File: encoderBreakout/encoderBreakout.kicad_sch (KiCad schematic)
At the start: 2 parts, among them J1 Conn_01x08_MountingPin

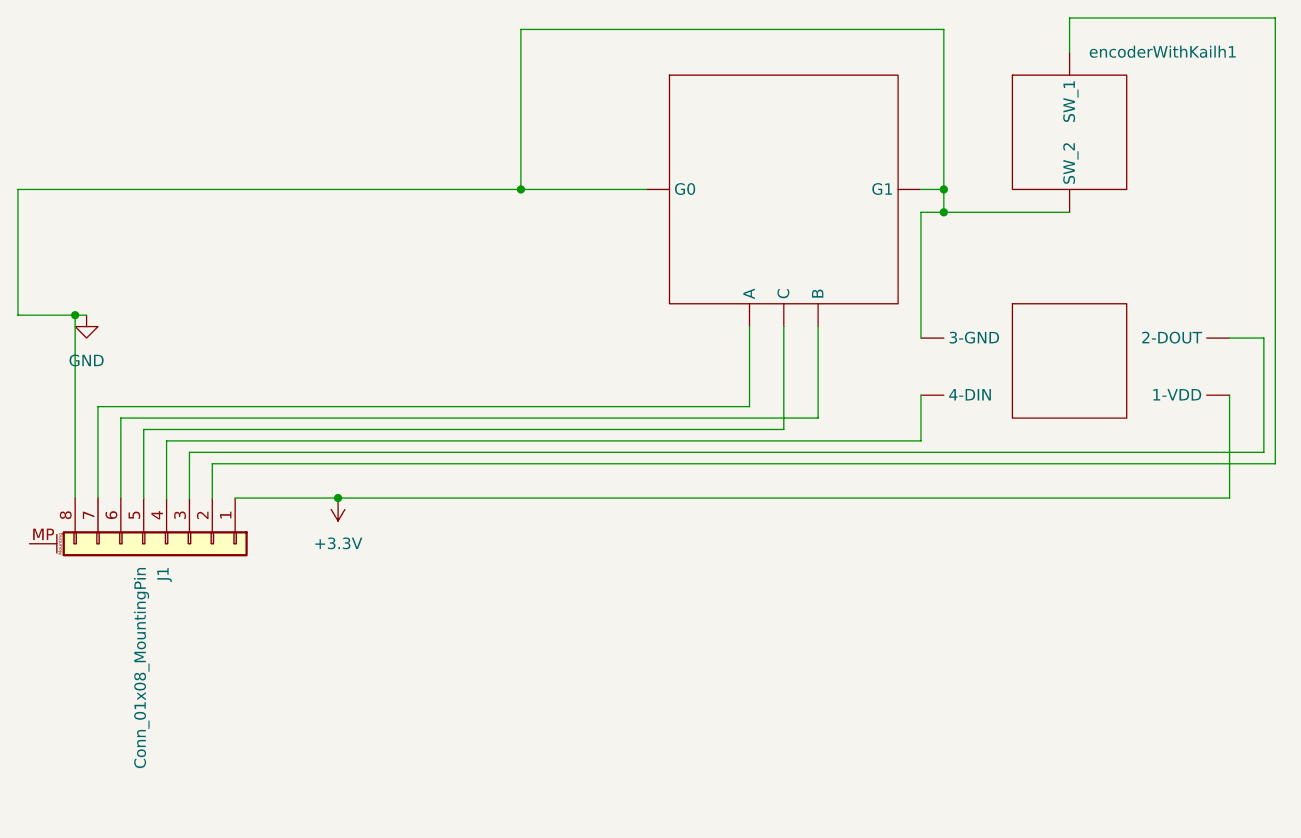
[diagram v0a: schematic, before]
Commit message: encoder breakout rev a
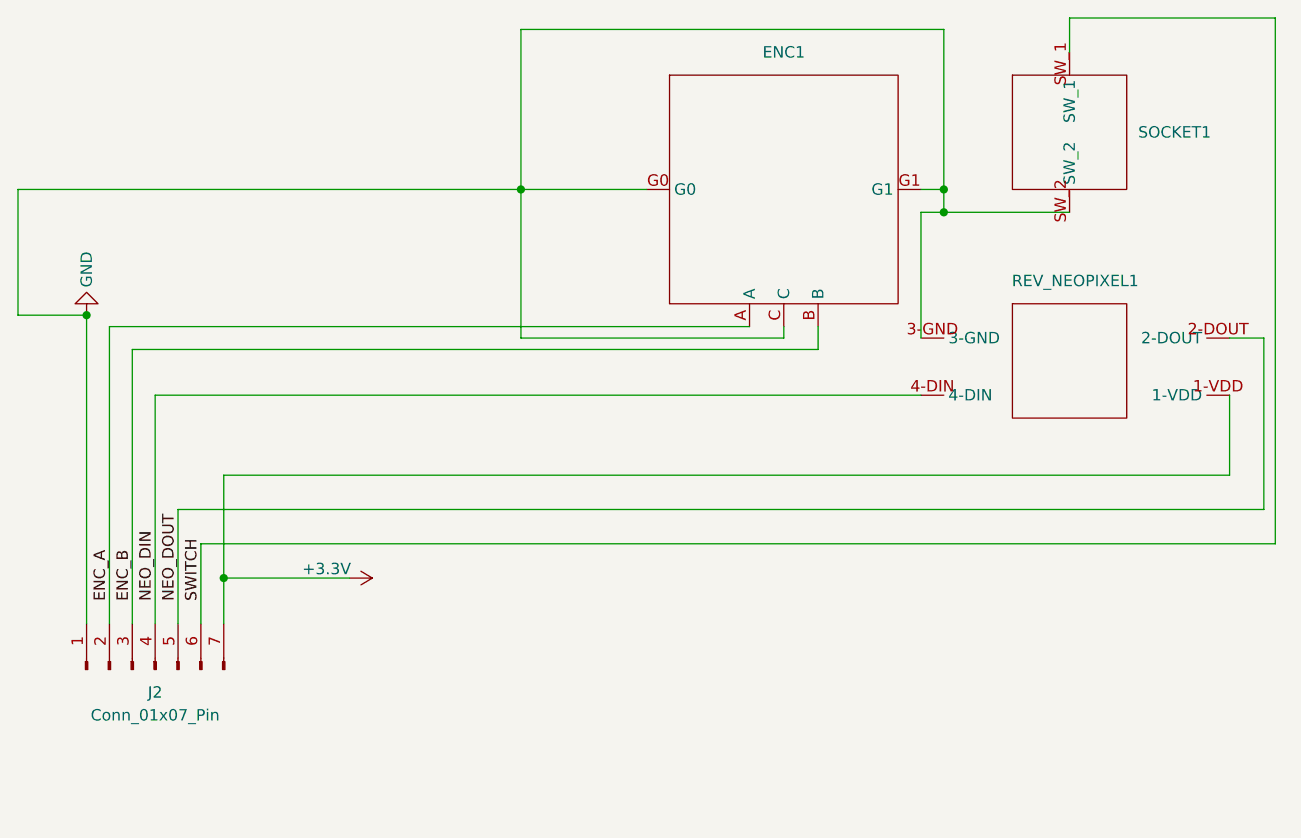
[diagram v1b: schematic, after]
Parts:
- removed J1: Conn_01x08_MountingPin, Connector_PinSocket_2.54mm:PinSocket_1x08_P2.54mm_Vertical, symbol Connector_Generic_MountingPin:Conn_01x08_MountingPin
- removed encoderWithKailh1: (no value), encLibrary:EC35AwithKailhSocket, symbol encSymbols:encoderWithKailh
- added ENC1: (no value), blitz_lib:EC35A_nosocket, symbol encSymbols:encoder
- added J2: Conn_01x07_Pin, Connector_PinHeader_2.54mm:PinHeader_1x07_P2.54mm_Vertical, symbol Connector:Conn_01x07_Pin
- added REV_NEOPIXEL1: (no value), blitz_lib:reverse_neopixel, symbol encSymbols:reverseNeopixel
- added SOCKET1: (no value), blitz_lib:kailh_socket, symbol encSymbols:kailhSocket
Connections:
- net +3.3V: now also J2.7 (Pin_7), REV_NEOPIXEL1.1-VDD
- net GND: now also ENC1.C, ENC1.G0, ENC1.G1, J2.1 (Pin_1), REV_NEOPIXEL1.3-GND, SOCKET1.SW_2
- new net ENC_A: ENC1.A, J2.2 (Pin_2)
- new net ENC_B: ENC1.B, J2.3 (Pin_3)
- new net NEO_DIN: J2.4 (Pin_4), REV_NEOPIXEL1.4-DIN
- new net NEO_DOUT: J2.5 (Pin_5), REV_NEOPIXEL1.2-DOUT
- new net SWITCH: J2.6 (Pin_6), SOCKET1.SW_1
